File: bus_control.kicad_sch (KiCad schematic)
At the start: 14 parts, among them U24 74LS138, U30 74LS32, U31 74LS32, U40 74LS138, U41 74LS00, U42 74LS08, U45 74LS138

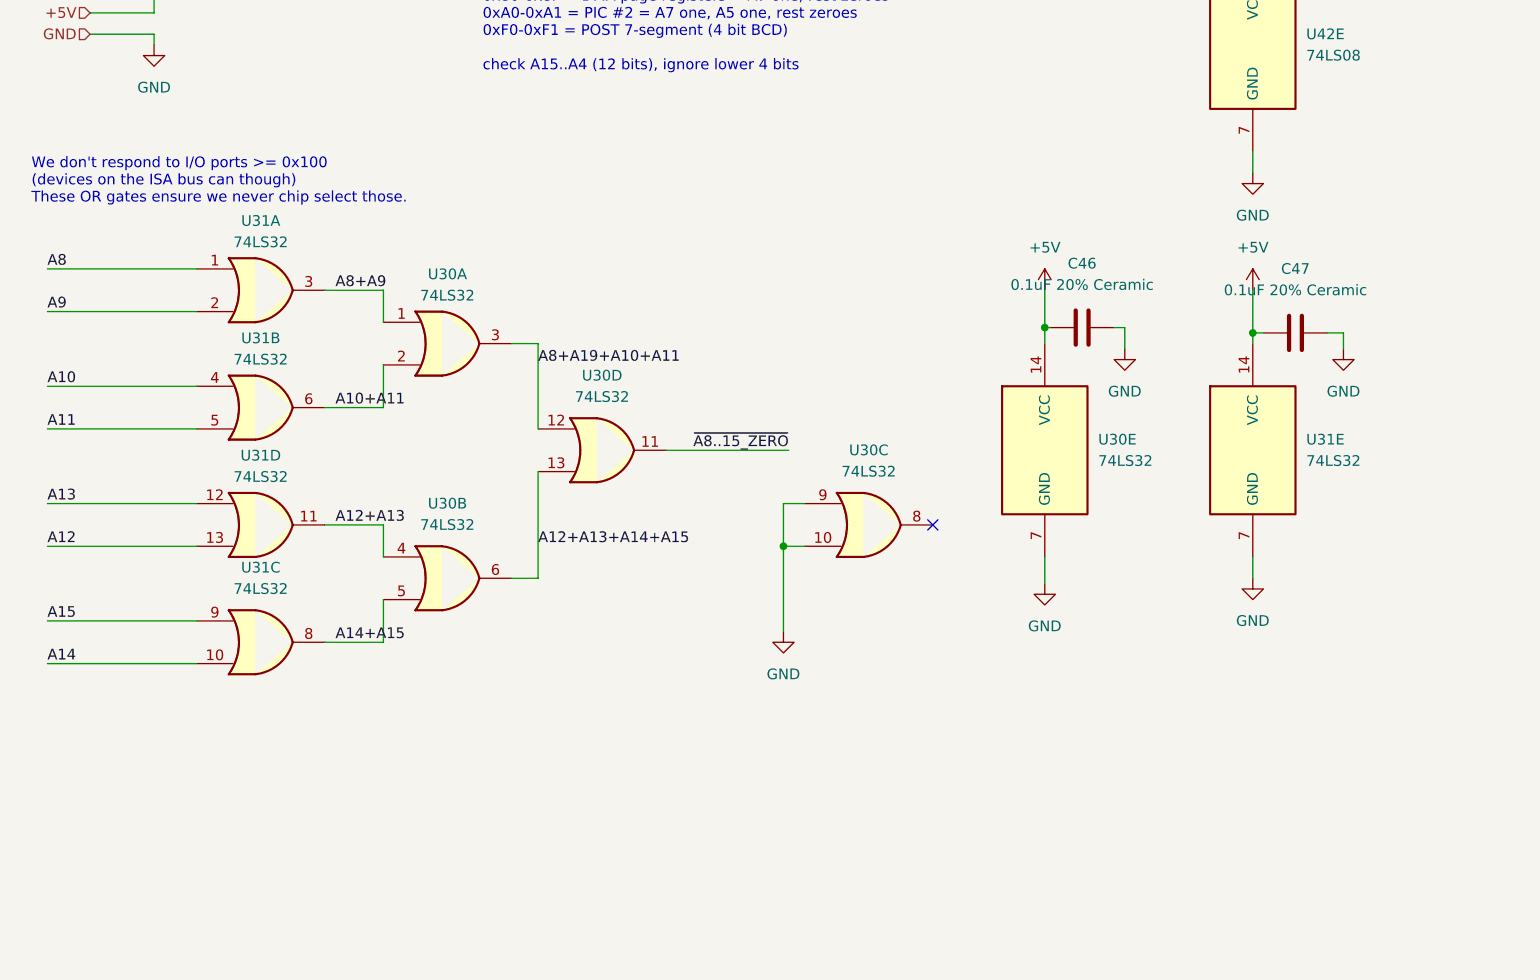
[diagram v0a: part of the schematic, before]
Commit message: routing tweaks, use identity comparator instead of OR gates for IO decode
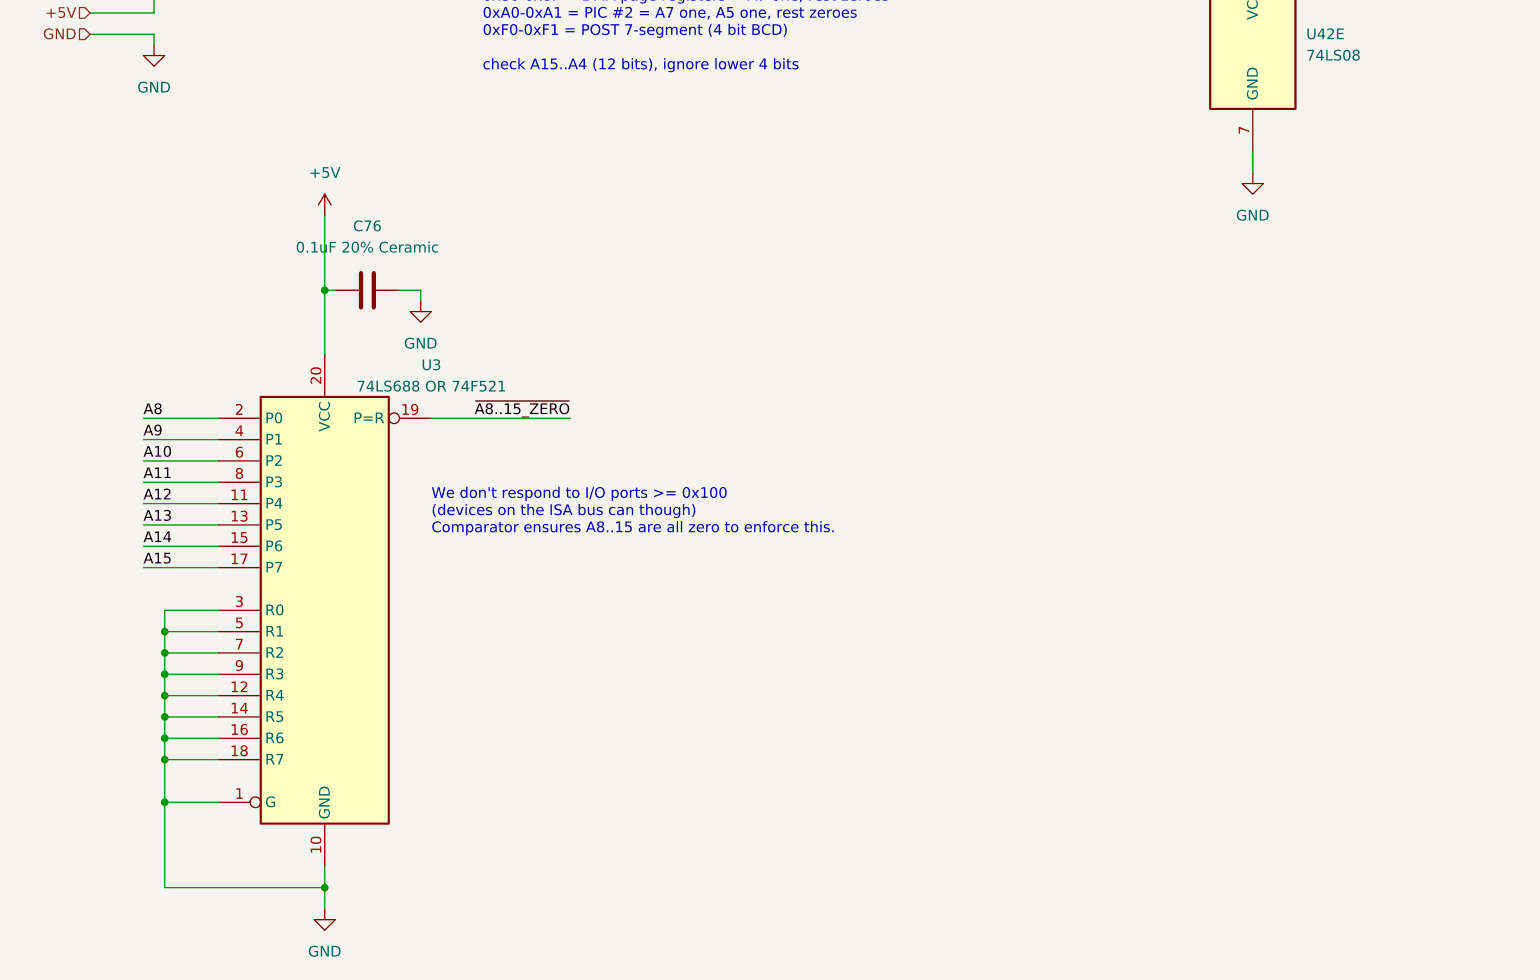
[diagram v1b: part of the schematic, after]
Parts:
- removed C46, C47: 0.1uF 20% Ceramic, Capacitor_SMD:C_0805_2012Metric, symbol Device:C
- removed U30, U31: 74LS32, Package_DIP:DIP-14_W7.62mm_Socket, symbol 74xx:74LS32
- added C76: 0.1uF 20% Ceramic, Capacitor_SMD:C_0805_2012Metric, symbol Device:C
- added U3: 74LS688 OR 74F521, Package_DIP:DIP-20_W7.62mm_Socket, symbol 74xx:74LS688
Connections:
- net +5V: now also C76.1, U3.20 (VCC)
- net A10: now also U3.6 (P2)
- net A11: now also U3.8 (P3)
- net A12: now also U3.11 (P4)
- net A13: now also U3.13 (P5)
- net A14: now also U3.15 (P6)
- net A15: now also U3.17 (P7)
- net A8: now also U3.2 (P0)
- net A9: now also U3.4 (P1)
- net GND: now also C76.2, U3.1 (G), U3.10 (GND), U3.12 (R4), U3.14 (R5), U3.16 (R6), U3.18 (R7), U3.3 (R0), U3.5 (R1), U3.7 (R2), U3.9 (R3)
- net ~{A8..15_ZERO}: now also U3.19 (P=R)
- no-connect marks 10 -> 9
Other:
- note added: "We don't respond to I/O ports >= 0x100 (devices on the ISA bus can though) Comparator ensures A8..15 are all zero to enforce this."
- note removed: "We don't respond to I/O ports >= 0x100 (devices on the ISA bus can though) These OR gates ensure we never chip select those."
